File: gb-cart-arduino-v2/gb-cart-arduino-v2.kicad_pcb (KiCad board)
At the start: 2 copper layers, 57.5 x 55 mm, 18 parts, among them J1 Conn_01x16_Pin, U1 74HC595, U2 74HC595

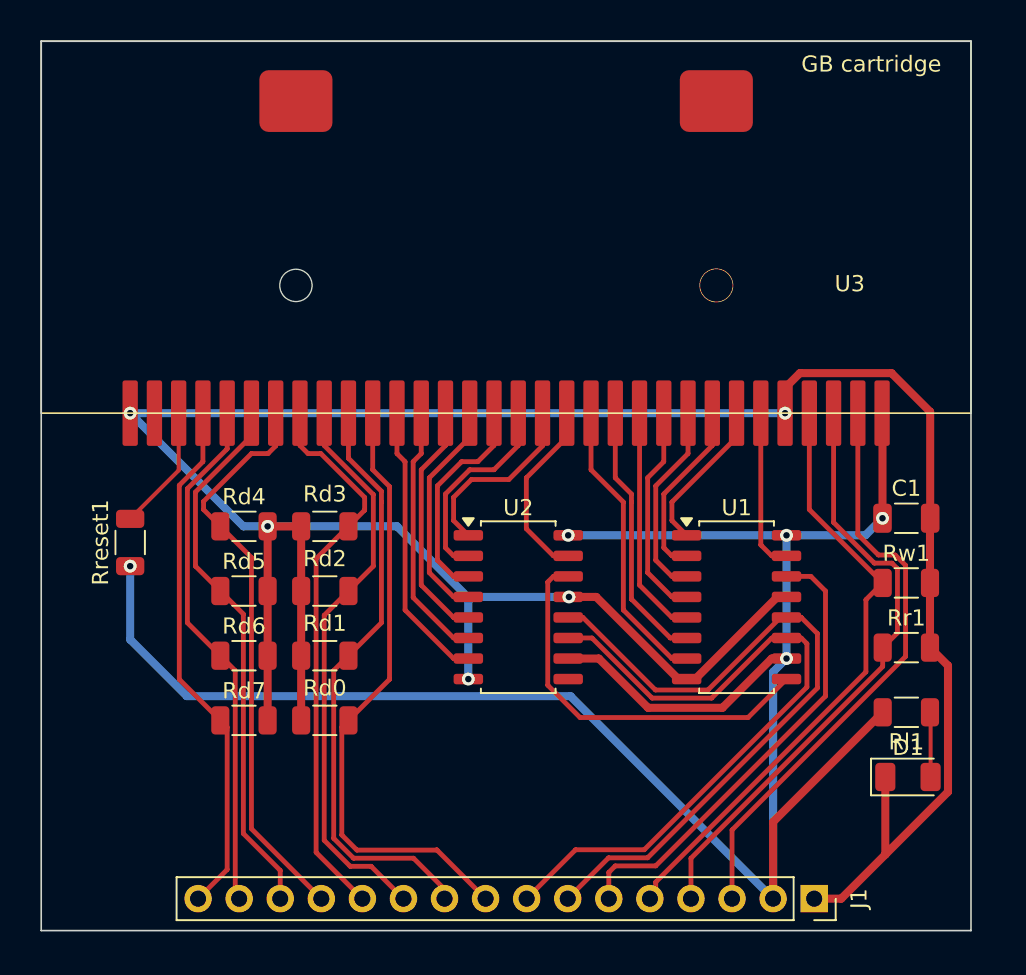
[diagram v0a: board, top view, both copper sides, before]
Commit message: Update
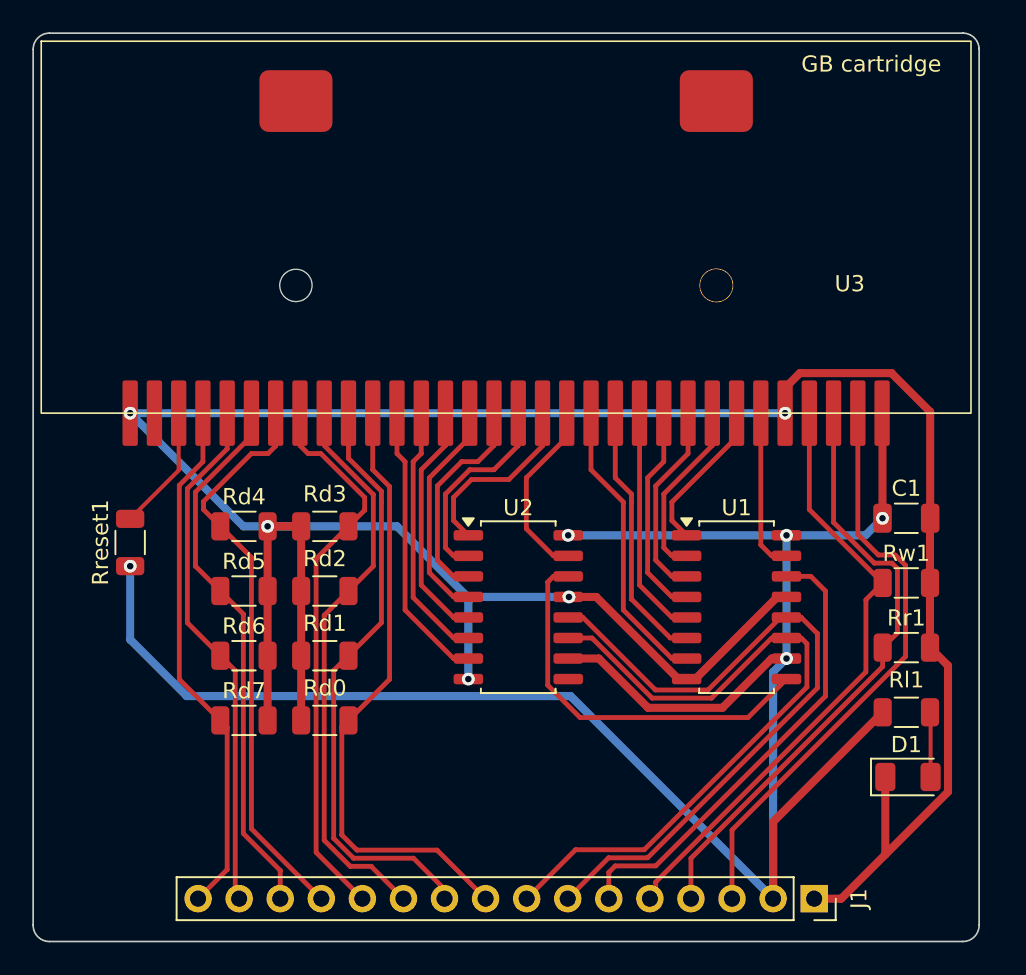
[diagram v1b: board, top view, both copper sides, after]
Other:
- board size 57.5 x 55 mm -> 58.5 x 56.2 mm
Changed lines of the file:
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@@
 		(tags "resistor")
 		(property "Reference" "Rl1"
-			(at 0 -1.83 0)
+			(at 0 2 0)
 			(layer "F.SilkS")
 			(effects
@@
 		(tags "LED")
 		(property "Reference" "D1"
-			(at 0 -1.83 0)
+			(at -0.1 -2 0)
 			(layer "F.SilkS")
 			(effects
@@
 		)
 	)
-	(gr_rect
-		(start 97 66.5)
-		(end 154.5 121.5)
+	(gr_line
+		(start 97.5 66)
+		(end 154 66)
+		(stroke
+			(width 0.1)
+			(type default)
+		)
+		(layer "Edge.Cuts")
+	)
+	(gr_line
+		(start 96.5 121.175)
+		(end 96.5 67)
+		(stroke
+			(width 0.1)
+			(type default)
+		)
+		(layer "Edge.Cuts")
+	)
+	(gr_line
+		(start 154 122.175)
+		(end 97.5 122.175)
+		(stroke
+			(width 0.1)
+			(type default)
+		)
+		(layer "Edge.Cuts")
+	)
+	(gr_arc
+		(start 155 121.175)
+		(mid 154.707107 121.882107)
+		(end 154 122.175)
+		(stroke
+			(width 0.1)
+			(type default)
+		)
+		(layer "Edge.Cuts")
+	)
+	(gr_arc
+		(start 97.5 122.175)
+		(mid 96.792893 121.882107)
+		(end 96.5 121.175)
+		(stroke
+			(width 0.1)
+			(type default)
+		)
+		(layer "Edge.Cuts")
+	)
+	(gr_line
+		(start 155 67)
+		(end 155 121.175)
+		(stroke
+			(width 0.1)
+			(type default)
+		)
+		(layer "Edge.Cuts")
+	)
+	(gr_arc
+		(start 154 66)
+		(mid 154.707107 66.292893)
+		(end 155 67)
+		(stroke
+			(width 0.1)
+			(type default)
+		)
+		(layer "Edge.Cuts")
+	)
+	(gr_arc
+		(start 96.5 67)
+		(mid 96.792893 66.292893)
+		(end 97.5 66)
 		(stroke
 			(width 0.1)
 			(type default)
 		)
-		(fill no)
 		(layer "Edge.Cuts")
 	)
@@
 	)
 	(segment
-		(start 118.0385 95.001)
-		(end 118.0375 95)
-		(width 0.3)
-		(layer "F.Cu")
-		(net 7)
-	)
-	(segment
 		(start 116.314979 117.0235)
 		(end 115.0865 115.795021)
@@
 	)
 	(segment
-		(start 121.4775 116.5225)
-		(end 121.455 116.5)
-		(width 0.3)
-		(layer "F.Cu")
-		(net 10)
-	)
-	(segment
 		(start 115.5875 108.9125)
 		(end 116 108.5)
@@
 		(width 0.3)
 		(layer "F.Cu")
-		(net 22)
-	)
-	(segment
-		(start 133.501 95.001)
-		(end 133.502 95)
-		(width 0.3)
-		(layer "F.Cu")
